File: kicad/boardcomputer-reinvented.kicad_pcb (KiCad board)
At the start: 2 copper layers, 55 x 60 mm, 0 parts

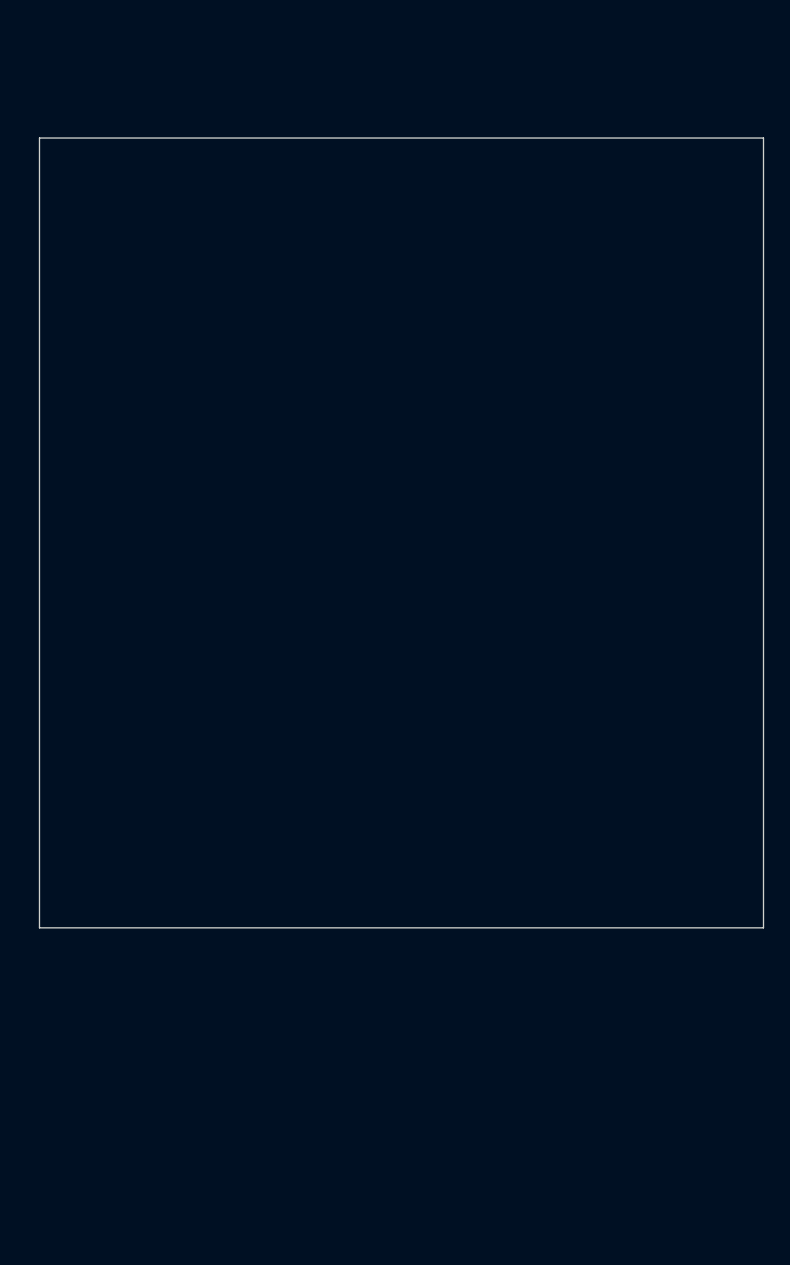
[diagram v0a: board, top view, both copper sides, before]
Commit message: Finished routing
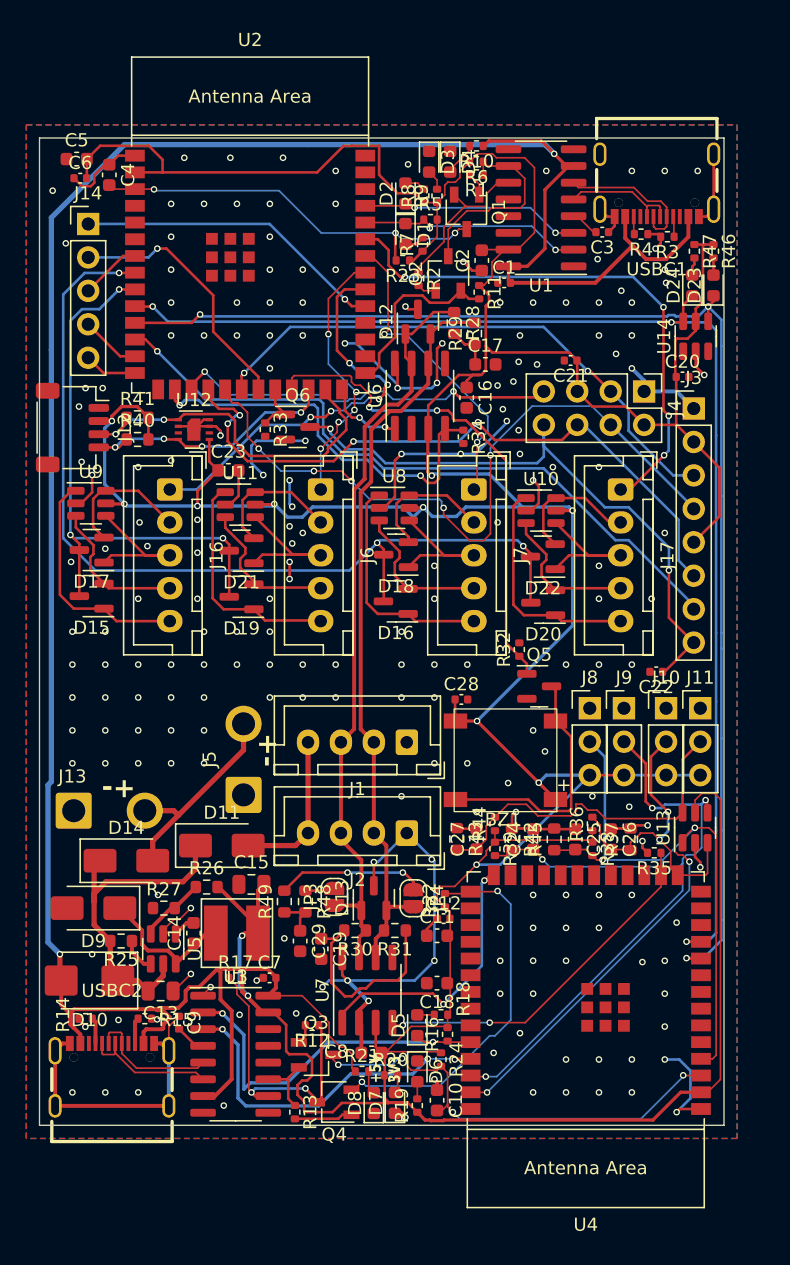
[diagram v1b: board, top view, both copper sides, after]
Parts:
- added BZ1: Buzzer, boardcomputer:Buzzer, F.Cu at (55.4, 67.3)
- added C1: 100n, Capacitor_SMD:C_0402_1005Metric, F.Cu at (55.3, 31.0)
- added C10: 10u, Capacitor_SMD:C_0603_1608Metric, F.Cu at (50.2, 93.1)
- added C11: 10u, Capacitor_SMD:C_0603_1608Metric, F.Cu at (50.2, 80.6)
- added C12: 100n, Capacitor_SMD:C_0402_1005Metric, F.Cu at (50.7, 79.3)
- added C13: 22uF, Capacitor_SMD:C_0805_2012Metric, F.Cu at (29.2, 84.8)
- added C14: 10n, Capacitor_SMD:C_0603_1608Metric, F.Cu at (31.7, 80.4)
- added C15: 22uF, Capacitor_SMD:C_0805_2012Metric, F.Cu at (36.1, 76.7)
- added C16: 100n, Capacitor_SMD:C_0603_1608Metric, F.Cu at (52.5, 39.7)
- added C17: 100n, Capacitor_SMD:C_0603_1608Metric, F.Cu at (53.9, 37.2)
- added C18: 100n, Capacitor_SMD:C_0603_1608Metric, F.Cu at (50.2, 84.2)
- added C19: 100n, Capacitor_SMD:C_0603_1608Metric, F.Cu at (41.4, 81.6)
- added C2: 1u, Capacitor_SMD:C_0603_1608Metric, F.Cu at (53.6, 29.3)
- added C20: 100n, Capacitor_SMD:C_0402_1005Metric, F.Cu at (68.8, 38.1)
- added C21: 100n, Capacitor_SMD:C_0402_1005Metric, F.Cu at (60.4, 36.9)
- added C22: 100n, Capacitor_SMD:C_0402_1005Metric, F.Cu at (66.8, 60.5)
- added C23: 100nF, Capacitor_SMD:C_0603_1608Metric, F.Cu at (34.4, 45.2)
- added C24: 100n, Capacitor_SMD:C_0603_1608Metric, F.Cu at (57.5, 73.3)
- added C25: 100n, Capacitor_SMD:C_0603_1608Metric, F.Cu at (60.7, 73.3)
- added C26: 100n, Capacitor_SMD:C_0603_1608Metric, F.Cu at (63.4, 73.3)
- added C27: 100n, Capacitor_SMD:C_0603_1608Metric, F.Cu at (53.2, 73.2)
- added C28: 100n, Capacitor_SMD:C_0402_1005Metric, F.Cu at (52.0, 62.6)
- added C29: 100nF, Capacitor_SMD:C_0603_1608Metric, F.Cu at (39.8, 81.0)
- added C3: 100n, Capacitor_SMD:C_0402_1005Metric, F.Cu at (62.8, 27.1)
- added C4: 10u, Capacitor_SMD:C_0603_1608Metric, F.Cu at (25.3, 22.8)
- added C5: 10u, Capacitor_SMD:C_0603_1608Metric, F.Cu at (22.8, 21.6)
- added C6: 100n, Capacitor_SMD:C_0402_1005Metric, F.Cu at (23.1, 23.1)
- added C7: 100n, Capacitor_SMD:C_0402_1005Metric, F.Cu at (37.5, 83.8)
- added C8: 1u, Capacitor_SMD:C_0603_1608Metric, F.Cu at (45.2, 89.5)
- added C9: 100n, Capacitor_SMD:C_0402_1005Metric, F.Cu at (30.6, 87.2)
- added D1: LED, LED_SMD:LED_0603_1608Metric, F.Cu at (47.8, 27.3)
- added D10: D, Diode_SMD:D_SMB, F.Cu at (23.8, 84.0)
- added D11: B230A, Diode_SMD:D_SMA, F.Cu at (33.9, 73.8)
- added D12: NUP2105L, Package_TO_SOT_SMD:SOT-23, F.Cu at (48.8, 34.0)
- added D13: NUP2105L, Package_TO_SOT_SMD:SOT-23, F.Cu at (45.4, 77.7)
- added D14: B230A, Diode_SMD:D_SMA, F.Cu at (26.6, 74.9)
- added D15: BAV99, Package_TO_SOT_SMD:SOT-23, F.Cu at (24.0, 54.8)
- added D16: BAV99, Package_TO_SOT_SMD:SOT-23, F.Cu at (47.1, 55.2)
- added D17: BAV99, Package_TO_SOT_SMD:SOT-23, F.Cu at (24.0, 51.3)
- added D18: BAV99, Package_TO_SOT_SMD:SOT-23, F.Cu at (47.1, 51.6)
- added D19: BAV99, Package_TO_SOT_SMD:SOT-23, F.Cu at (35.4, 54.9)
- added D2: LED, LED_SMD:LED_0603_1608Metric, F.Cu at (47.8, 24.2)
- added D20: BAV99, Package_TO_SOT_SMD:SOT-23, F.Cu at (58.3, 55.3)
- added D21: BAV99, Package_TO_SOT_SMD:SOT-23, F.Cu at (35.4, 51.4)
- added D22: BAV99, Package_TO_SOT_SMD:SOT-23, F.Cu at (58.2, 51.8)
- added D23: LED, LED_SMD:LED_0603_1608Metric, F.Cu at (71.2, 31.2)
- added D24: LED, LED_SMD:LED_0603_1608Metric, F.Cu at (69.6, 31.2)
- added D3: LED, LED_SMD:LED_0603_1608Metric, F.Cu at (49.6, 21.8)
- added D4: LED5V, LED_SMD:LED_0603_1608Metric, F.Cu at (51.2, 21.8)
- added D5: LED, LED_SMD:LED_0603_1608Metric, F.Cu at (48.7, 87.4)
- added D6: LED, LED_SMD:LED_0603_1608Metric, F.Cu at (48.7, 90.9)
- added D7: LED, LED_SMD:LED_0603_1608Metric, F.Cu at (47.0, 93.3)
- added D8: LED5V, LED_SMD:LED_0603_1608Metric, F.Cu at (45.4, 93.3)
- added D9: B230A, Diode_SMD:D_SMA, F.Cu at (24.1, 78.5)
- added J1: CAN1, Connector_JST:JST_XH_B4B-XH-A_1x04_P2.50mm_Vertical, F.Cu at (47.9, 65.9)
- added J10: BREMSE, Connector_PinHeader_2.54mm:PinHeader_1x03_P2.54mm_Vertical, F.Cu at (67.6, 63.3)
- added J11: BREMSE, Connector_PinHeader_2.54mm:PinHeader_1x03_P2.54mm_Vertical, F.Cu at (70.2, 63.3)
- added J12: I2C, Connector_JST:JST_SH_SM04B-SRSS-TB_1x04-1MP_P1.00mm_Horizontal, F.Cu at (22.5, 42.0)
- added J13: Conn_01x02_Pin, Connector_Wire:SolderWire-1sqmm_1x02_P5.4mm_D1.4mm_OD2.7mm, F.Cu at (22.6, 71.1)
- added J14: Conn_01x05_Pin, Connector_PinHeader_2.54mm:PinHeader_1x05_P2.54mm_Vertical, F.Cu at (23.7, 26.5)
- added J16: BUTTON1, Connector_JST:JST_XH_B5B-XH-A_1x05_P2.50mm_Vertical, F.Cu at (29.9, 46.7)
- added J17: BUTTON4, Connector_JST:JST_XH_B5B-XH-A_1x05_P2.50mm_Vertical, F.Cu at (64.2, 46.7)
- added J2: CAN2, Connector_JST:JST_XH_B4B-XH-A_1x04_P2.50mm_Vertical, F.Cu at (47.9, 72.8)
- added J3: Conn_Display, Connector_PinHeader_2.54mm:PinHeader_1x08_P2.54mm_Vertical, F.Cu at (69.7, 40.5)
- added J4: Conn_Display, Connector_PinHeader_2.54mm:PinHeader_2x04_P2.54mm_Vertical, F.Cu at (65.9, 39.2)
- added J5: Conn_01x02_Pin, Connector_Wire:SolderWire-1sqmm_1x02_P5.4mm_D1.4mm_OD2.7mm, F.Cu at (35.5, 69.9)
- added J6: BUTTON2, Connector_JST:JST_XH_B5B-XH-A_1x05_P2.50mm_Vertical, F.Cu at (41.4, 46.7)
- added J7: BUTTON3, Connector_JST:JST_XH_B5B-XH-A_1x05_P2.50mm_Vertical, F.Cu at (53.0, 46.7)
- added J8: GAS, Connector_PinHeader_2.54mm:PinHeader_1x03_P2.54mm_Vertical, F.Cu at (61.8, 63.3)
- added J9: GAS, Connector_PinHeader_2.54mm:PinHeader_1x03_P2.54mm_Vertical, F.Cu at (64.4, 63.3)
- added JP3: SolderJumper_2_Open, Jumper:SolderJumper-2_P1.3mm_Open_RoundedPad1.0x1.5mm, F.Cu at (42.4, 77.7)
- added JP4: SolderJumper_2_Open, Jumper:SolderJumper-2_P1.3mm_Open_RoundedPad1.0x1.5mm, F.Cu at (48.4, 77.7)
- added L1: 4.7uH, boardcomputer:L_5040, F.Cu at (35.0, 80.4)
- added Q1: SS8050_C2150, Package_TO_SOT_SMD:TSOT-23, F.Cu at (52.5, 25.6)
- added Q2: SS8050_C2150, Package_TO_SOT_SMD:TSOT-23, F.Cu at (51.0, 30.3)
- added Q3: SS8050_C2150, Package_TO_SOT_SMD:TSOT-23, F.Cu at (41.0, 89.6)
- added Q4: SS8050_C2150, Package_TO_SOT_SMD:TSOT-23, F.Cu at (42.4, 93.2)
- added Q5: 2N7002, Package_TO_SOT_SMD:SOT-23, F.Cu at (58.0, 61.7)
- added Q6: 2N7002, Package_TO_SOT_SMD:SOT-23, F.Cu at (39.6, 42.0)
- added R1: 12k, Resistor_SMD:R_0402_1005Metric, F.Cu at (53.2, 22.8)
- added R10: 1k, Resistor_SMD:R_0402_1005Metric, F.Cu at (53.2, 20.6)
- added R11: 1k, Resistor_SMD:R_0402_1005Metric, F.Cu at (53.4, 31.7)
- added R12: 12k, Resistor_SMD:R_0402_1005Metric, F.Cu at (40.7, 87.4)
- added R13: 12k, Resistor_SMD:R_0402_1005Metric, F.Cu at (39.4, 94.0)
- added R14: 5k1, Resistor_SMD:R_0402_1005Metric, F.Cu at (23.5, 86.9)
- added R15: 5k1, Resistor_SMD:R_0402_1005Metric, F.Cu at (28.0, 86.9)
- added R16: 10k, Resistor_SMD:R_0402_1005Metric, F.Cu at (51.0, 88.1)
- added R17: 10k, Resistor_SMD:R_0402_1005Metric, F.Cu at (34.9, 83.8)
- added R18: 1k, Resistor_SMD:R_0402_1005Metric, F.Cu at (50.5, 86.6)
- added R19: 1k, Resistor_SMD:R_0402_1005Metric, F.Cu at (48.7, 93.5)
- added R2: 12k, Resistor_SMD:R_0402_1005Metric, F.Cu at (48.8, 30.7)
- added R20: 1k, Resistor_SMD:R_0402_1005Metric, F.Cu at (46.7, 91.2)
- added R21: 1k, Resistor_SMD:R_0402_1005Metric, F.Cu at (44.5, 90.9)
- added R22: 1k, Resistor_SMD:R_0402_1005Metric, F.Cu at (50.8, 77.9)
- added R23: 1k, Resistor_SMD:R_0402_1005Metric, F.Cu at (47.6, 29.3)
- added R24: 1k, Resistor_SMD:R_0402_1005Metric, F.Cu at (50.5, 90.0)
- added R25: 1k, Resistor_SMD:R_0603_1608Metric, F.Cu at (26.2, 81.0)
- added R26: 49.9k, Resistor_SMD:R_0603_1608Metric, F.Cu at (32.7, 76.9)
- added R27: 16.2k, Resistor_SMD:R_0603_1608Metric, F.Cu at (29.4, 78.5)
- added R28: 56R, Resistor_SMD:R_0603_1608Metric, F.Cu at (51.5, 34.0)
- added R29: 56R, Resistor_SMD:R_0603_1608Metric, F.Cu at (53.0, 34.9)
- added R3: 5k1, Resistor_SMD:R_0402_1005Metric, F.Cu at (67.7, 27.5)
- added R30: 56R, Resistor_SMD:R_0603_1608Metric, F.Cu at (44.0, 80.2)
- added R31: 56R, Resistor_SMD:R_0603_1608Metric, F.Cu at (47.0, 80.2)
- added R32: 10k, Resistor_SMD:R_0402_1005Metric, F.Cu at (56.5, 58.9)
- added R33: 10k, Resistor_SMD:R_0402_1005Metric, F.Cu at (37.1, 42.1)
- added R34: 1k, Resistor_SMD:R_0402_1005Metric, F.Cu at (52.2, 42.7)
- added R35: 1k, Resistor_SMD:R_0402_1005Metric, F.Cu at (66.7, 74.3)
- added R36: 10k, Resistor_SMD:R_0402_1005Metric, F.Cu at (62.0, 72.1)
- added R37: 100k, Resistor_SMD:R_0603_1608Metric, F.Cu at (64.9, 73.3)
- added R38: 10k, Resistor_SMD:R_0402_1005Metric, F.Cu at (62.0, 74.0)
- added R39: 10k, Resistor_SMD:R_0402_1005Metric, F.Cu at (54.6, 74.0)
- added R4: 5k1, Resistor_SMD:R_0402_1005Metric, F.Cu at (65.7, 27.3)
- added R40: 2k2, Resistor_SMD:R_0603_1608Metric, F.Cu at (27.4, 42.9)
- added R41: 2k2, Resistor_SMD:R_0603_1608Metric, F.Cu at (27.4, 41.2)
- added R42: 100k, Resistor_SMD:R_0603_1608Metric, F.Cu at (55.9, 73.3)
- added R43: 100k, Resistor_SMD:R_0603_1608Metric, F.Cu at (51.7, 73.3)
- added R44: 10k, Resistor_SMD:R_0402_1005Metric, F.Cu at (54.6, 72.1)
- added R45: 100k, Resistor_SMD:R_0603_1608Metric, F.Cu at (59.1, 73.3)
- added R46: 1k, Resistor_SMD:R_0402_1005Metric, F.Cu at (71.2, 28.6)
- added R47: 1k, Resistor_SMD:R_0402_1005Metric, F.Cu at (69.8, 28.6)
- added R48: 56, Resistor_SMD:R_0603_1608Metric, F.Cu at (40.2, 78.0)
- added R49: 56, Resistor_SMD:R_0603_1608Metric, F.Cu at (38.6, 78.0)
- added R5: 10k, Resistor_SMD:R_0402_1005Metric, F.Cu at (49.7, 26.2)
- added R6: 10k, Resistor_SMD:R_0402_1005Metric, F.Cu at (53.2, 21.8)
- added R7: 1k, Resistor_SMD:R_0402_1005Metric, F.Cu at (49.1, 28.1)
- added R8: 1k, Resistor_SMD:R_0402_1005Metric, F.Cu at (49.2, 24.4)
- added R9: 1k, Resistor_SMD:R_0402_1005Metric, F.Cu at (50.2, 24.4)
- added U1: CH343G, Package_SO:SOIC-16_3.9x9.9mm_P1.27mm, F.Cu at (58.1, 25.3)
- added U10: USBLC6-4SC6, Package_TO_SOT_SMD:SOT-23-6, F.Cu at (58.1, 48.3)
- added U11: USBLC6-4SC6, Package_TO_SOT_SMD:SOT-23-6, F.Cu at (35.2, 47.9)
- added U12: SHT30-DIS, Sensor_Humidity:Sensirion_DFN-8-1EP_2.5x2.5mm_P0.5mm_EP1.1x1.7mm, F.Cu at (31.7, 42.1)
- added U13: USBLC6-4SC6, Package_TO_SOT_SMD:SOT-23-6, F.Cu at (69.8, 72.4)
- added U14: USBLC6-4SC6, Package_TO_SOT_SMD:SOT-23-6, F.Cu at (69.9, 35.1)
- added U2: ESP32-S3-WROOM-1-ENTERTAINMENT, PCM_Espressif:ESP32-S3-WROOM-1, F.Cu at (36.0, 29.6)
- added U3: CH343G, Package_SO:SOIC-16_3.9x9.9mm_P1.27mm, F.Cu at (34.9, 89.6)
- added U4: ESP32-S3-WROOM-1-CONTROL, PCM_Espressif:ESP32-S3-WROOM-1, F.Cu at (61.5, 85.5)
- added U5: MPM2359, Package_TO_SOT_SMD:SOT-23-6, F.Cu at (29.4, 81.6)
- added U6: SN65HVD231, Package_SO:SOIC-8_3.9x4.9mm_P1.27mm, F.Cu at (48.9, 39.6)
- added U7: SN65HVD231, Package_SO:SOIC-8_3.9x4.9mm_P1.27mm, F.Cu at (44.9, 84.7)
- added U8: USBLC6-4SC6, Package_TO_SOT_SMD:SOT-23-6, F.Cu at (47.0, 48.1)
- added U9: USBLC6-4SC6, Package_TO_SOT_SMD:SOT-23-6, F.Cu at (23.9, 47.8)
- added USBC1: MC-311D, usb_c:USB-C-SMD_MC-311D, F.Cu at (66.9, 23.6)
- added USBC2: MC-311D, usb_c:USB-C-SMD_MC-311D, F.Cu at (25.5, 91.2)
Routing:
- net +3.3V: track 0.00 -> 386.8 mm, vias 0 -> 12
- net +5V: track 0.00 -> 191.4 mm, vias 0 -> 2
- net GND: track 0.00 -> 169.7 mm, vias 0 -> 206
- net PROCESSOR_COMMUNICATION_CONTROLESP_TX: track 0.00 -> 99.3 mm, vias 0 -> 3
- net PROCESSOR_COMMUNICATION_CONTROLESP_RX: track 0.00 -> 97.5 mm, vias 0 -> 3
- net OUT2: track 0.00 -> 71.0 mm, vias 0 -> 3
- net CANH: track 0.00 -> 57.9 mm
- net CANL: track 0.00 -> 57.1 mm
- net RAW_M365_BREMSE: track 0.00 -> 56.6 mm, vias 0 -> 2
- net RAW_M365_GAS: track 0.00 -> 56.3 mm, vias 0 -> 4
- net DISPLAY_MOSI: track 0.00 -> 53.6 mm, vias 0 -> 5
- net DISPLAY_CS1: track 0.00 -> 52.4 mm, vias 0 -> 1
- net DISPLAY_DC: track 0.00 -> 51.0 mm, vias 0 -> 4
- net Net-(J3-Pin_8): track 0.00 -> 47.3 mm, vias 0 -> 2
- net OUT1: track 0.00 -> 43.4 mm, vias 0 -> 3
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- added copper zone on B.Cu, net GND
- added copper zone on F.Cu, net GND
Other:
- board size 55 x 60 mm -> 52 x 75 mm
- board text added: "+-"
- board text added: "+5V 3V3"
